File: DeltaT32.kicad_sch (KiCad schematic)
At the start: 35 parts, among them J1 PH2.0, J2 USB_C_Receptacle_USB2.0_16P, J3 SH1.0, Q1 AO3401A, SW1 Boot, SW2 Reset, SW3 SW_SPDT_312, U1 TP4057, U2 MPU-6050, U3 ESP32-C3-MINI-1, U4 AP2112K-3.3

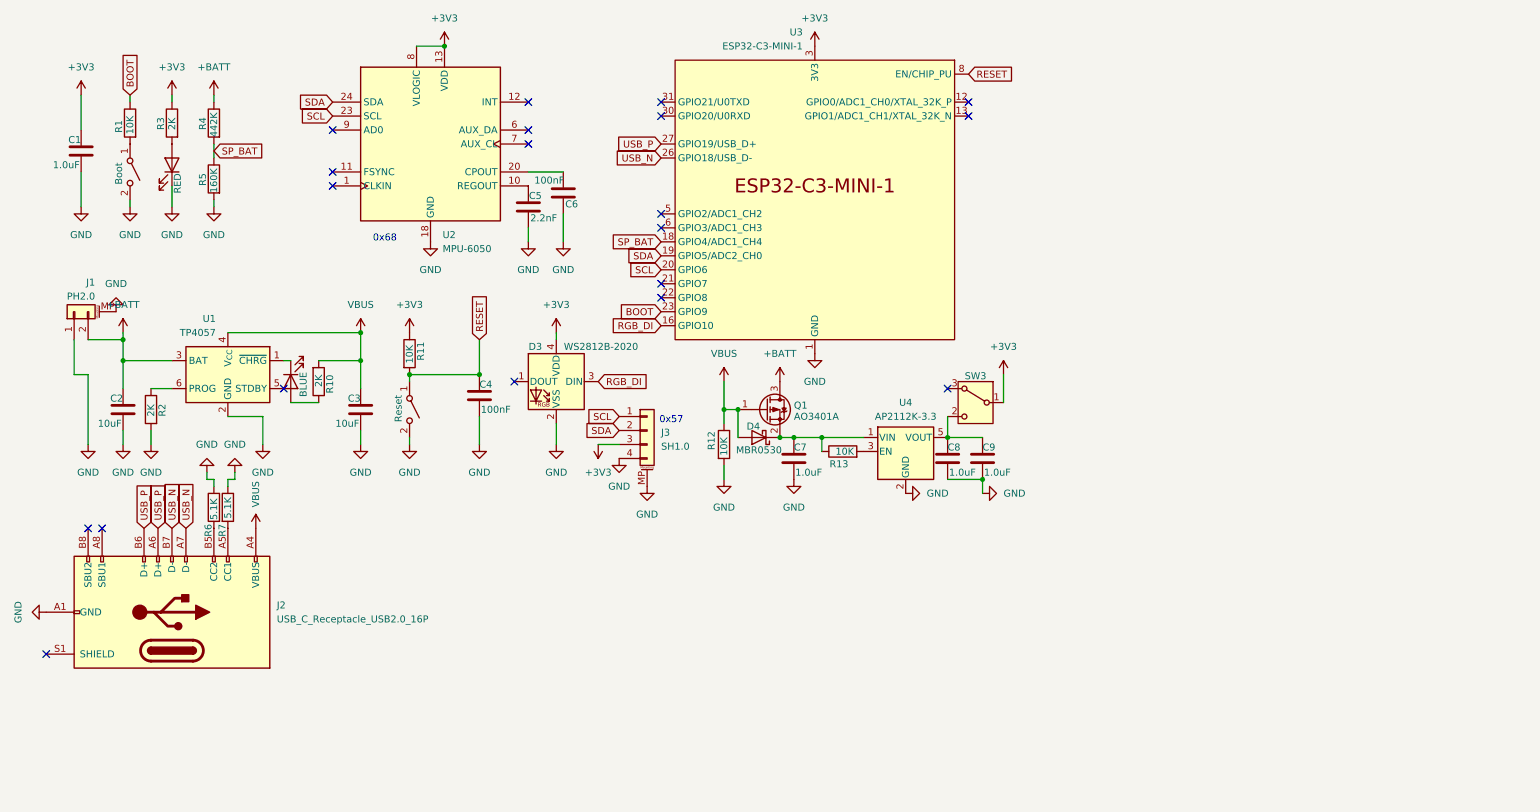
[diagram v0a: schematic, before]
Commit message: Update Board
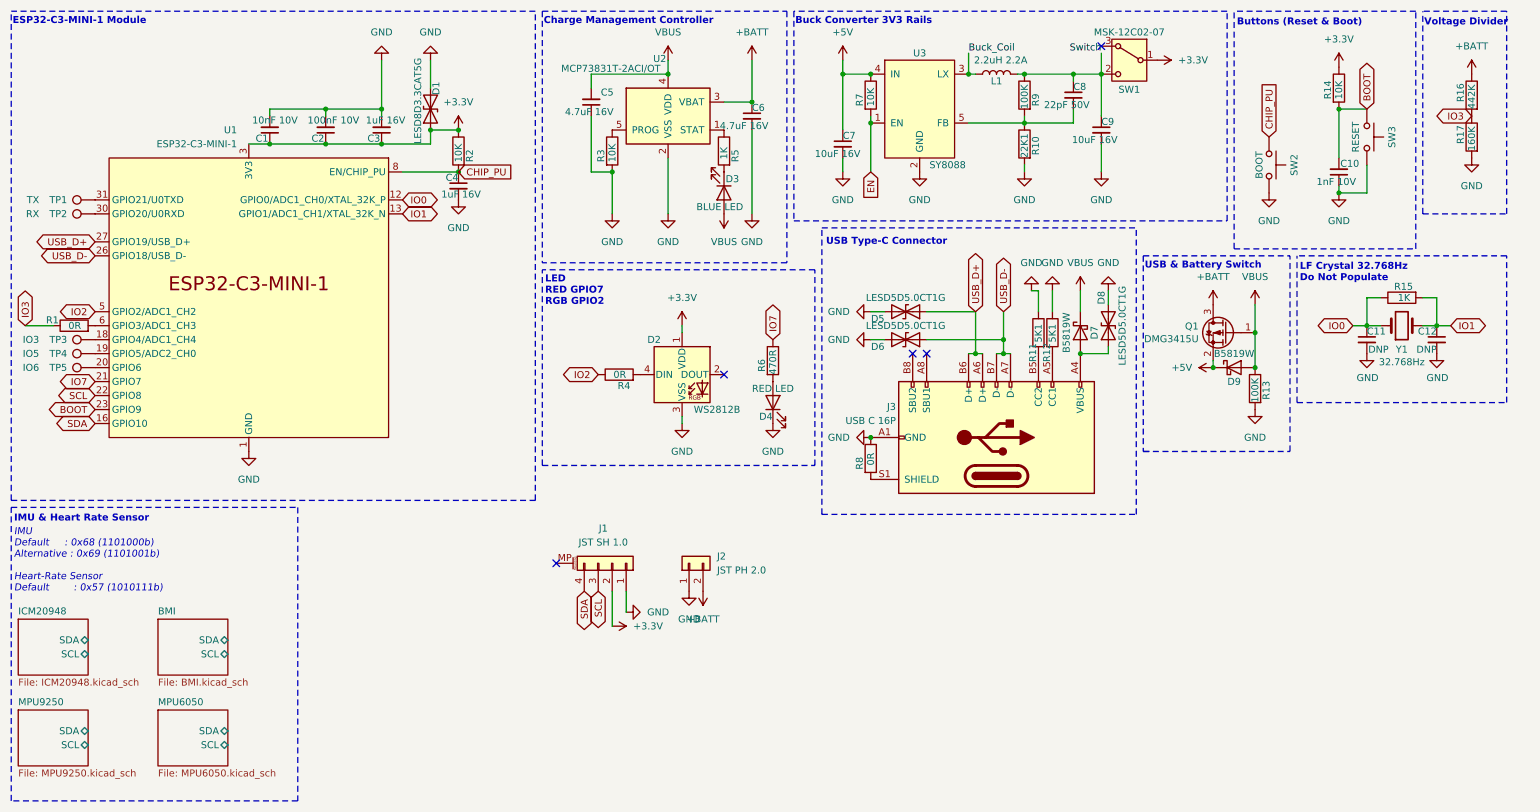
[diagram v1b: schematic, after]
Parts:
- removed C1, C7, C8, C9: 1.0uF, Capacitor_SMD:C_0402_1005Metric, symbol Device:C
- removed C2, C3: 10uF, Capacitor_SMD:C_0402_1005Metric, symbol Device:C
- removed C4, C6: 100nF, Capacitor_SMD:C_0402_1005Metric, symbol Device:C
- removed C5: 2.2nF, Capacitor_SMD:C_0603_1608Metric, symbol Device:C
- removed D1: RED, LED_SMD:LED_0402_1005Metric, symbol Device:LED
- removed D2: BLUE, LED_SMD:LED_0402_1005Metric, symbol Device:LED
- removed D3: WS2812B-2020, LED_SMD:LED_WS2812B-2020_PLCC4_2.0x2.0mm, symbol LED:WS2812B-2020
- removed D4: MBR0530, Diode_SMD:D_SOD-123, symbol Diode:MBR0530
- removed J1: PH2.0, Connector_JST:JST_PH_B2B-PH-SM4-TB_1x02-1MP_P2.00mm_Vertical, symbol Connector_Generic_MountingPin:Conn_01x02_MountingPin
- removed J3: SH1.0, Connector_JST:JST_SH_BM04B-SRSS-TB_1x04-1MP_P1.00mm_Vertical, symbol Connector_Generic_MountingPin:Conn_01x04_MountingPin
- removed Q1: AO3401A, Package_TO_SOT_SMD:SOT-23, symbol Transistor_FET:AO3401A
- removed R11, R12: 10K, Resistor_SMD:R_0402_1005Metric, symbol Device:R
- removed SW1: Boot, Button_Switch_SMD:SW_Push_SPST_NO_Alps_SKRK, symbol Switch:SW_SPST
- removed SW2: Reset, Button_Switch_SMD:SW_Push_SPST_NO_Alps_SKRK, symbol Switch:SW_SPST
- removed SW3: SW_SPDT_312, Button_Switch_SMD:SW_SPDT_PCM12, symbol Switch:SW_SPDT_312
- removed U1: TP4057, Package_TO_SOT_SMD:TSOT-23-6, symbol Battery_Management:TP4057
- removed U2: MPU-6050, Sensor_Motion:InvenSense_QFN-24_4x4mm_P0.5mm, symbol Sensor_Motion:MPU-6050
- removed U3: ESP32-C3-MINI-1, PCM_Espressif:ESP32-C3-MINI-1, symbol PCM_Espressif:ESP32-C3-MINI-1
- removed U4: AP2112K-3.3, Package_TO_SOT_SMD:SOT-23-5, symbol Regulator_Linear:AP2112K-3.3
- added C1: 10nF 10V, Capacitor_SMD:C_0402_1005Metric, symbol Device:C_Small
- added C10: 1nF 10V, Capacitor_SMD:C_0402_1005Metric, symbol Device:C_Small
- added C11, C12: DNP, Capacitor_SMD:C_0402_1005Metric, symbol Device:C_Small
- added C2: 100nF 10V, Capacitor_SMD:C_0402_1005Metric, symbol Device:C_Small
- added C3, C4: 1uF 16V, Capacitor_SMD:C_0402_1005Metric, symbol Device:C_Small
- added C5, C6: 4.7uF 16V, Capacitor_SMD:C_0603_1608Metric, symbol Device:C_Small
- added C7, C9: 10uF 16V, Capacitor_SMD:C_0805_2012Metric, symbol Device:C_Small
- added C8: 22pF 50V, Capacitor_SMD:C_0603_1608Metric, symbol Device:C_Small
- added D1: LESD8D3.3CAT5G, Diode_SMD:D_SOD-882, symbol Device:D_TVS
- added D2: WS2812B, LED_SMD:LED_WS2812B-2020_PLCC4_2.0x2.0mm, symbol LED:WS2812B
- added D3: BLUE LED, LED_SMD:LED_0603_1608Metric, symbol Device:LED
- added D4: RED LED, LED_SMD:LED_0603_1608Metric, symbol Device:LED
- added D5, D6, D8: LESD5D5.0CT1G, Diode_SMD:D_SOD-523, symbol Device:D_TVS
- added D7, D9: B5819W, Diode_SMD:D_SOD-123, symbol Device:D_Schottky
- added J1: JST SH 1.0, Connector_JST:JST_SH_SM04B-SRSS-TB_1x04-1MP_P1.00mm_Horizontal, symbol Connector_Generic_MountingPin:Conn_01x04_MountingPin
- added J2: JST PH 2.0, Connector_JST:JST_PH_B2B-PH-K_1x02_P2.00mm_Vertical, symbol Connector_Generic:Conn_01x02
- added L1: 2.2uH 2.2A, Inductor_SMD:L_Bourns-SRN4018, symbol Device:L
- added Q1: DMG3415U, Package_TO_SOT_SMD:SOT-23, symbol Transistor_FET:DMG2301L
- added R14, R7: 10K, Resistor_SMD:R_0402_1005Metric, symbol Device:R
- added R15, R5: 1K, Resistor_SMD:R_0402_1005Metric, symbol Device:R
- added R4, R8: 0R, Resistor_SMD:R_0402_1005Metric, symbol Device:R
- added R6: 470R, Resistor_SMD:R_0402_1005Metric, symbol Device:R
- added R9: 100K, Resistor_SMD:R_0402_1005Metric, symbol Device:R
- added SW1: MSK-12C02-07, Button_Switch_SMD:SW_SPDT_PCM12, symbol Switch:SW_SPDT_312
- added SW2: BOOT, Button_Switch_SMD:SW_Push_SPST_NO_Alps_SKRK, symbol Switch:SW_Push
- added SW3: RESET, Button_Switch_SMD:SW_Push_SPST_NO_Alps_SKRK, symbol Switch:SW_Push
- added TP1: TX, TestPoint:TestPoint_Pad_D1.0mm, symbol Connector:TestPoint
- added TP2: RX, TestPoint:TestPoint_Pad_D1.0mm, symbol Connector:TestPoint
- added TP3: IO3, TestPoint:TestPoint_Pad_D1.0mm, symbol Connector:TestPoint
- added TP4: IO5, TestPoint:TestPoint_Pad_D1.0mm, symbol Connector:TestPoint
- added TP5: IO6, TestPoint:TestPoint_Pad_D1.0mm, symbol Connector:TestPoint
- added U1: ESP32-C3-MINI-1, PCM_Espressif:ESP32-C3-MINI-1, symbol PCM_Espressif:ESP32-C3-MINI-1
- added U2: MCP73831T-2ACI/OT, Package_TO_SOT_SMD:SOT-23-5, symbol Battery_Management:MCP73831-2-OT
- added U3: SY8088, Package_TO_SOT_SMD:SOT-23-5, symbol Rust_Board:SY8088
- added Y1: 32.768Hz, Crystal:Crystal_SMD_3215-2Pin_3.2x1.5mm, symbol Device:Crystal
- J3: renamed from J2; value USB_C_Receptacle_USB2.0_16P -> USB C 16P; footprint Connector_USB:USB_C_Receptacle_GCT_USB4110 -> Connector_USB:USB_C_Receptacle_GCT_USB4105-xx-A_16P_TopMnt_Horizontal
- R1: value 10K -> 0R
- R10: value 2K -> 22K1
- R11: renamed from R6; value 5.1K -> 5K1
- R12: renamed from R7; value 5.1K -> 5K1
- R13: value 10K -> 100K
- R2, R3: value 2K -> 10K
- renumbered R4 to R16, R5 to R17
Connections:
- net +BATT: now also C6.1, J2.2 (Pin_2), Q1.3 (D), U2.3 (VBAT)
- net BOOT: now also C10.2, R14.2, SW3.1, U1.23 (GPIO9); no longer R1.1
- net GND: now also R10.2, R13.2, R3.2, C1.2, C10.1, C11.2, C12.2, C2.2, C3.2, C4.2, C5.1, C6.2, C7.2, C9.2, D1.2 (A2), D2.3 (VSS), D4.1 (K), D5.2 (A2), D6.2 (A2), D8.2 (A2), J1.1 (Pin_1), J2.1 (Pin_1), R8.1, SW2.2, SW3.2, U1.1 (GND), U1.11 (GND), U1.14 (GND), U1.2 (GND), U1.36 (GND), U1.37 (GND), U1.38 (GND), U1.39 (GND), U1.40 (GND), U1.41 (GND), U1.42 (GND), U1.43 (GND), U1.44 (GND), U1.45 (GND), U1.46 (GND), U1.47 (GND), U1.48 (GND), U1.49 (GND), U1.50 (GND), U1.51 (GND), U1.52 (GND), U1.53 (GND), U2.2 (VSS), U3.2 (GND); no longer R2.2
- net SCL: now also J1.3 (Pin_3), U1.22 (GPIO8)
- net SDA: now also J1.4 (Pin_4), U1.16 (GPIO10)
- net VBUS: now also R13.1, C5.2, D3.2 (A), D7.1 (K), D9.2 (A), Q1.1 (G), U2.4 (VDD); no longer J3.A4 (VBUS), J3.A9 (VBUS), J3.B4 (VBUS), J3.B9 (VBUS), R10.2
- net +3.3V: now reaches R2.1
- net +3.3V: now also C1.1, C2.1, C3.1, D1.1 (A1), D2.1 (VDD), J1.2 (Pin_2), R14.1, SW1.1 (B), U1.3 (3V3)
- net at R1.2: now also U1.6 (GPIO3/ADC1_CH3)
- net at R10.1: now also C8.2, R9.2, U3.5 (FB)
- net at J3.S1 (SHIELD): now also R8.2
- net +3V3: no longer names the net of R3.1
- net +3V3: now also U2.5 (PROG)
- net SP_BAT renamed IO3
- net IO3: now also R1.1
- net USB_N renamed USB_D-
- net USB_D-: now also D6.1 (A1), U1.26 (GPIO18/USB_D-)
- net USB_P renamed USB_D+
- net USB_D+: now also D5.1 (A1), U1.27 (GPIO19/USB_D+)
- new net: TP3.1, U1.18 (GPIO4/ADC1_CH4)
- new net: R5.1, U2.1 (STAT)
- new net: D3.1 (K), R5.2
- new net: D7.2 (A), D8.1 (A1), J3.A4 (VBUS), J3.A9 (VBUS), J3.B4 (VBUS), J3.B9 (VBUS)
- new net: D2.4 (DIN), R4.2
- new net: TP4.1, U1.19 (GPIO5/ADC2_CH0)
- new net: TP5.1, U1.20 (GPIO6)
- new net: TP2.1, U1.30 (GPIO20/U0RXD)
- new net: TP1.1, U1.31 (GPIO21/U0TXD)
- new net: D4.2 (A), R6.2
- new net +5V: C7.1, D9.1 (K), Q1.2 (S), R7.1, U3.4 (IN)
- new net Buck_Coil: L1.1, U3.3 (LX)
- new net CHIP_PU: C4.1, R2.2, SW2.1, U1.8 (EN/CHIP_PU)
- new net EN: R7.2, U3.1 (EN)
- new net IO0: C11.1, R15.1, U1.12 (GPIO0/ADC1_CH0/XTAL_32K_P), Y1.1
- new net IO1: C12.1, R15.2, U1.13 (GPIO1/ADC1_CH1/XTAL_32K_N), Y1.2
- new net IO2: R4.1, U1.5 (GPIO2/ADC1_CH2)
- new net IO7: R6.1, U1.21 (GPIO7)
- new net Switch: C8.1, C9.1, L1.2, R9.1, SW1.2 (C)
- no-connect marks 20 -> 5
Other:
- added sheet BMI (BMI.kicad_sch)
- added sheet ICM20948 (ICM20948.kicad_sch)
- added sheet MPU6050 (MPU6050.kicad_sch)
- added sheet MPU9250 (MPU9250.kicad_sch)
- note added: "Buck Converter 3V3 Rails"
- note added: "Buttons (Reset & Boot)"
- note added: "Charge Management Controller"
- note added: "ESP32-C3-MINI-1 Module"
- note added: "IMU & Heart Rate Sensor"
- note added: "IMU Default : 0x68 (1101000b) Alternative : 0x69 (1101001b) Heart-Rate Sensor Default : 0x57 (1010111b)"
- note added: "LED RED GPIO7 RGB GPIO2"
- note added: "LF Crystal 32.768Hz Do Not Populate"
- note added: "USB & Battery Switch"
- note added: "USB Type-C Connector"
- note added: "Voltage Divider"
- title: (none) -> DeltaT32
- moved on the sheet: J3, R11, R12, R16, R17

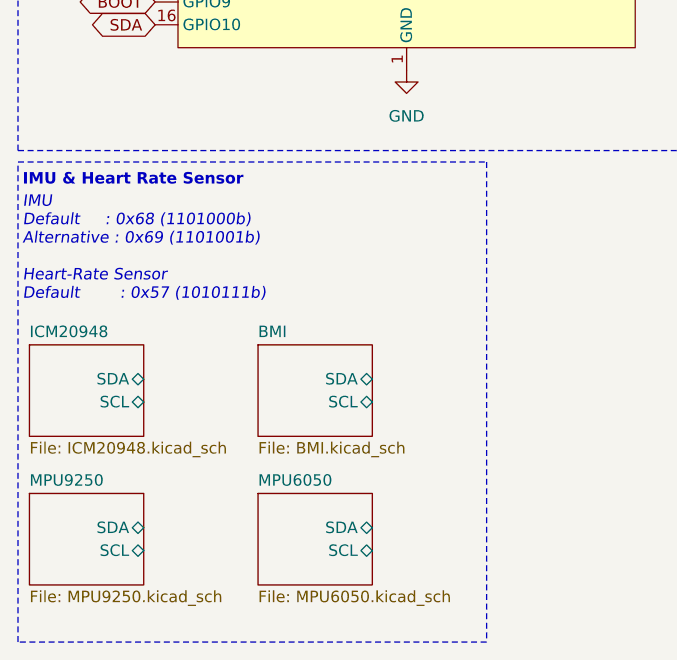
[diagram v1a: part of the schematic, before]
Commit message: Update Board
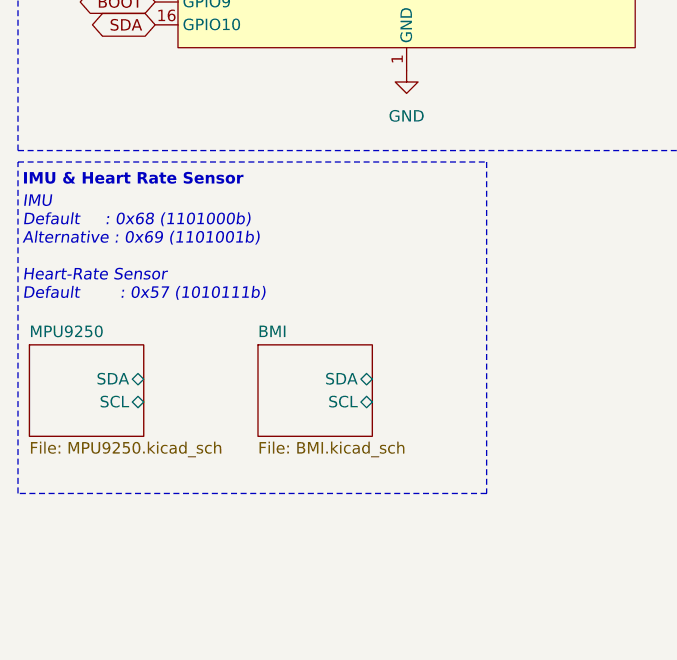
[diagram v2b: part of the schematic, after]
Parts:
- J2: footprint Connector_JST:JST_PH_B2B-PH-K_1x02_P2.00mm_Vertical -> Connector_JST:JST_PH_S2B-PH-K_1x02_P2.00mm_Horizontal
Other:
- removed sheet ICM20948
- removed sheet MPU6050
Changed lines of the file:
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@@
 	(polyline
 		(pts
-			(xy 64.77 102.87) (xy 64.77 156.21)
+			(xy 64.77 102.87) (xy 64.77 139.7)
 		)
 		(stroke
@@
 	(polyline
 		(pts
-			(xy 12.7 156.21) (xy 12.7 102.87)
+			(xy 12.7 139.7) (xy 12.7 102.87)
 		)
 		(stroke
@@
 	(polyline
 		(pts
-			(xy 64.77 156.21) (xy 12.7 156.21)
+			(xy 64.77 139.7) (xy 12.7 139.7)
 		)
 		(stroke
@@
 			"AAAAAAAAAAAAAAAAAAAAAAAAAAAAAAAAAAAAAAAAAAAAAAAAAAAAAADwAAAAAAAAAASzwJEABACA"
 			"0JgX/psBAACAvxj+mwEAAIC/GP6bAQAAABAAAAAAAAAAAAAAAAAAAICvGP6bAQAAAAAAAAAAAAAA"
-			"AAAAAAAAAAAAAAAAAAAAoK8Y/psBAAAAAAAAAAAAAAAAAAAAAAAAAAAAAAAAAADArxj+mw=="
+			"AAAAAAAAAAAAAAAAAAAAoK8Y/psBAAAAAAAAAAAAAAAAAAAAAAAAAAAAAAAAAADArxj+mwAAAAAA"
+			"AAAAAAAAAAAAAAAAAAAAAAAAAAAAAAAAAAAAAAAAAAAAAAAAAAAAAAAAAAAAAAAAAAAAAAAAAAAA"
+			"AAAAAAAAAAAAAAAAAAAAAAAAAAAAAAAAAAAAAAAAAAAAAAAAAAAAAAAAAAAAAAAAAAAAAAAAAAAA"
+			"AAAAAAAAAAAAAAAAAAAAAAAAAAAAAAAAAAAAAAAAAAAAAAAAAAAAAAAAAAAAAAAAAAAAAAAAAAAA"
+			"AAAAAAAAAAAAAAAAAAAAAAAAAAAAAAAAAAAAAAAAAAAAAAAAAAAAAAAAAAAAAAAAAAAAAAAAAAAA"
+			"AAAAAAAAAAAAAAAAAAAAAAAAAAAAAAAAAAAAAAAAAAAAAAAAAAAAAAAAAAAAAAAAAAAAAAAAAAAA"
+			"AAAAAAAAAAAAAAAAAAAAAAAAAAAAAAAAAAAAAAAAAAAAAAAAAAAAAAAAAAAAAAAAAAAAAAAAAAAA"
+			"AAAAAAAAAAAAAAAAAAAAAAAAAAAAAAAAAAAAAAAAAAAAAAAAAAAAAAAAAAAAAAAAAAAAAAAAAAAA"
+			"AAAAAAAAAAAAAAAAAAAAAAAAAAAAAAAAAAAAAAAAAAAAAAAAAAAAAAAAAAAAAAAAAAAAAAAAAAAA"
+			"AAAAAAAAAAAAAAAAAAAAAAAAAAAAAAAAAAAAAAAAAAAAAAAAAAAAAAAAAAAAAAAAAAAAAAAAAAAA"
+			"AAAAAAAAAAAAAAAAAAAAAAAAAAAAAAAAAAAAAAAAAAAAAAAAAAAAAAAAAAAAAAAAAAAAAAAAAAAA"
+			"AAAAAAAAAAAAAAAAAAAAAAAAAAAAAAAAAAAAAAAAAAAAAAAAAAAAAAAAAAAAAAAAAAAAAAAAAAAA"
+			"AAAAAAAAAAAAAAAAAAAAAAAAAAAAAAAAAAAAAAAAAAAAAAAAAAAAAAAAAAAAAAAAAAAAAAAAAAAA"
+			"AAAAAAAAAAAAAAAAAAAAAAAAAAAAAAAAAAAAAAAAAAAAAAAAAAAAAAAAAAAAAAAAAAAAAAAAAAAA"
+			"AAAAAAAAAAAAAAAAAAAAAAAAAAAAAAAAAAAAAAAAAAAAAAAAAAAAAAAAAAAAAAAAAAAAAAAAAAAA"
+			"AAAAAAAAAAAAAAAAAAAAAAAAAAAAAAAAAAAAAAAAAAAAAAAAAAAAAAAAAAAAAAAAAAAAAAAAAAAA"
+			"AAAAAAAAAAAAAAAAAAAAAAAAAAAAAAAAAAAAAAAAAAAAAAAAAAAAAAAAAAAAAAAAAAAAAAAAAAAA"
+			"AAAAAAAAAAAAAAAAAAAAAAAAAAAAAAAAAAAAAAAAAAAAAAAAAAAAAAAAAAAAAAAAAAAAAAAAAAAA"
+			"AAAAAAAAAAAAAAAAAAAAAAAAAAAAAAAAAAAAAAAAAAAAAAAAAAAAAAAAAAAAAAAAAAAAAAAAAAAA"
+			"AAAAAAAAAAAAAAAAAAAAAAAAAAAAAAAAAAAAAAAAAAAAAAAAAAAAAAAAAAAAAAAAAAAAAAAAAAAA"
+			"AAAAAAAAAAAAAAAAAAAAAAAAAAAAAAAAAAAAAAAAAAAAAAAAAAAAAAAAAAAAAAAAAAAAAAAAAAAA"
+			"AAAAAAAAAAAAAAAAAAAAAAAAAAAAAAAAAAAAAAAAAAAAAAAAAAAAAAAAAAAAAAAAAAAAAAAAAAAA"
+			"AAAAAAAAAAAAAAAAAAAAAAAAAAAAAAAAAAAAAAAAAAAAAAAAAAAAAAAAAAAAAAAAAAAAAAAAAAAA"
+			"AAAAAAAAAAAAAAAAAAAAAAAAAAAAAAAAAAAAAAAAAAAAAAAAAAAAAAAAAAAAAAAAAAAAAAAAAAAA"
+			"AAAAAAAAAAAAAAAAAAAAAAAAAAAAAAAAAAAAAAAAAAAAAAAAAAAAAAAAAAAAAAAAAAAAAAAAAAAA"
+			"AAAAAAAAAAAAAAAAAAAAAAAAAAAAAAAAAAAAAAAAAAAAAAAAAAAAAAAAAAAAAAAAAAAAAAAAAAAA"
+			"AAAAAAAAAAAAAAAAAAAAAAAAAAAAAAAAAAAAAAAAAAAAAAAAAAAAAAAAAAAAAAAAAAAAAAAAAAAA"
+			"AAAAAAAAAAAAAAAAAAAAAAAAAAAAAAAAAAAAAAAAAAAAAAAAAAAAAAAAAAAAAAAAAAAAAAAAAAAA"
+			"AAAAAAAAAAAAAAAAAAAAAAAAAAAAAAAAAAAAAAAAAAAAAAAAAAAAAAAAAAAAAAAAAAAAAAAAAAAA"
+			"AAAAAAAAAAAAAAAAAAAAAAAAAAAAAAAAAAAAAAAAAAAAAAAAAAAAAAAAAAAAAAAAAAAAAAAAAAAA"
+			"AAAAAAAAAAAAAAAAAAAAAAAAAAAAAAAAAAAAAAAAAAAAAAAAAAAAAAAAAAAAAAAAAAAAAAAAAAAA"
+			"AAAAAAAAAAAAAAAAAAAAAAAAAAAAAAAAAAAAAAAAAAAAAAAAAAAAAAAAAAAAAAAAAAAAAAAAAAAA"
+			"AAAAAAAAAAAAAAAAAAAAAAAAAAAAAAAAAAAAAAAAAAAAAAAAAAAAAAAAAAAAAAAAAAAAAAAAAAAA"
+			"AAAAAAAAAAAAAAAAAAAAAAAAAAAAAAAAAAAAAAAAAAAAAAAAAAAAAAAAAAAAAAAAAAAAAAAAAAAA"
+			"AAAAAAAAAAAAAAAAAAAAAAAAAAAAAAAAAAAAAAAAAAAAAAAAAAAAAAAAAAAAAAAAAAAAAAAAAAAA"
+			"AAAAAAAAAAAAAAAAAAAAAAAAAAAAAAAAAAAAAAAAAAAAAAAAAAAAAAAAAAAAAAAAAAAAAAAAAAAA"
+			"AAAAAAAAAAAAAAAAAAAAAAAAAAAAAAAAAAAAAAAAAAAAAAAAAAAAAAAAAAAAAAAAAAAAAP///wQA"
+			"AAD4/////////3gDAAAAAAAA/////wQAAAD4/////////wAAAAAAAAAA/////wQAAAD4////////"
+			"/94AAAAAAAAA/////wQAAAD4/////////98CAAAAAAAA/////wQAAAD4/////////2gBAAAAAAAA"
+			"/////wQAAAD4/////////wAAAAAAAAAA/////wQAAAD4/////////xsDAAAAAAAA/////wQAAAD4"
+			"/////////70AAAAAAAAA/////wQAAAD4/////////6IBAAAAAAAA/////wQAAAD4/////////9gA"
+			"AAAAAAAA/////wQAAAD4/////////w8BAAAAAAAA/////wQAAAD4/////////0EAAAAAAAAA////"
+			"/wQAAAD4/////////5oAAAAAAAAA/////wQAAAD4/////////wAAAAAAAAAA/////wQAAAD4////"
+			"/////wAAAAAAAAAA/////wQAAAD4/////////wAAAAAAAAAA/////wQAAAD4/////////5gAAAAA"
+			"AAAA/////wQAAAD4/////////wAAAAAAAAAA/////wQAAAD4/////////9ICAAAAAAAA/////wQA"
+			"AAD4/////////18AAAAAAAAA/////wQAAAD4/////////9kBAAAAAAAA/////wQAAAD4////////"
+			"/xwBAAAAAAAA/////wQAAAD4/////////0sAAAAAAAAA/////wQAAAD4/////////wAAAAAAAAAA"
+			"/////wQAAAD4/////////48AAAAAAAAA/////wQAAAD4/////////wAAAAAAAAAA/////wQAAAD4"
+			"/////////wAAAAAAAAAA/////wQAAAD4/////////wAAAAAAAAAA/////wQAAAD4/////////10A"
+			"AAAAAAAA/////wQAAAD4/////////5wAAAAAAAAA/////wQAAAD4/////////9gCAAAAAAAA////"
+			"/wQAAAD4/////////wAAAAAAAAAA/////wQAAAD4/////////wAAAAAAAAAA/////wQAAAD4////"
+			"/////wAAAAAAAAAA/////wQAAAD4/////////wAAAAAAAAAA/////wQAAAD4/////////wAAAAAA"
+			"AAAA/////wQAAAD4/////////zoBAAAAAAAA/////wQAAAD4/////////0sCAAAAAAAA/////wQA"
+			"AAD4/////////8wAAAAAAAAA/////wQAAAD4//////////kCAAAAAAAA/////wQAAAD4////////"
+			"/9QBAAAAAAAA/////wQAAAD4/////////wAAAAAAAAAA/////wQAAAD4/////////wAAAP9aWlr/"
+			"Wlpa/1paWv9aWlr/Wlpa/1paWv9aWlr/Wlpa/1paWv9aWlr/Wlpa/1paWv9aWlr/Wlpa/1paWv9a"
+			"Wlr/Wlpa/1paWv9aWlr/Wlpa/1paWv9aWlr/Wlpa/1paWv9aWlr/Wlpa/1paWv9aWlr/Wlpa/1pa"
+			"Wv9aWlr/Wlpa/1paWv9aWlr/Wlpa/1paWv9aWlr/Wlpa/1paWv9aWlr/Wlpa/1paWv9aWlr/Wlpa"
+			"/1paWv9aWlr/Wlpa/1paWv9aWlr/Wlpa/1paWv9aWlr/Wlpa/1paWv+inIz/0MWs/9DFrP/Qxaz/"
+			"0MWs/9DFrP/Qxaz/0MWs/9DFrP/Qxaz/0MWs/9DFrP/Qxaz/0MWs/9DFrP/Qxaz/0MWs/9DFrP/Q"
+			"xaz/0MWs/9DFrP/Qxaz/0MWs/9DFrP/Qxaz/0MWs/9DFrP/Qxaz/0MWs/9DFrP/Qxaz/0MWs/9DF"
+			"rP/Qxaz/0MWs/9DFrP/Qxaz/0MWs/9DFrP/Qxaz/0MWs/9DFrP/Qxaz/0MWs/9DFrP/Qxaz/0MWs"
+			"/9DFrP/Qxaz/0MWs/9DFrP/Qxaz/0MWs/9DFrP/Qxaz/0MWs/9DFrP/Qxaz/0MWs/9DFrP/Qxaz/"
+			"0MWs/9DFrP/Qxaz/0MWs/9DFrP/Qxaz/0MWs/9DFrP/Qxaz/0MWs/9DFrP/Qxaz/0MWs/9DFrP/Q"
+			"xaz/0MWs/9DFrP/Qxaz/0MWs/9DFrP/Qxaz/0MWs/9DFrP/Qxaz/0MWs/9DFrP/Qxaz/0MWs/9DF"
+			"rP/Qxaz/0MWs/9DFrP/Qxaz/0MWs/9DFrP/Qxaz/0MWs/9DFrP/Qxaz/0MWs/9DFrP/Qxaz/0MWs"
+			"/9DFrP/Qxaz/0MWs/9DFrP/Qxaz/0MWs/9DFrP/Qxaz/0MWs/9DFrP/Qxaz/0MWs/9DFrP/Qxaz/"
+			"0MWs/9DFrP/Qxaz/0MWs/9DFrP/Qxaz/0MWs/9DFrP/Qxaz/vbOd/zMzM/8zMzP/MzMz/zMzM/8z"
+			"MzP/MzMz/zMzM/8zMzP/MzMz/zMzM/8zMzP/MzMz/zMzM/8zMzP/MzMz/zMzM/8zMzP/MzMz/zMz"
+			"M/8zMzP/MzMz/zMzM/8zMzP/SUdE/6CZh//Qxaz/0MWs/9DFrP/Qxaz/0MWs/9DFrP/Qxaz/0MWs"
+			"/9DFrP/Qxaz/0MWs/9DFrP/Qxaz/0MWs/9DFrP/Topv/4RBS/9wfV//gFlT/0L+p/9DFrP/Qxaz/"
+			"0MWs/9DFrP/Qxaz/0MWs/9DFrP/Qxaz/0MWs/9DFrP/Qxaz/0MWs/9DFrP/Qxaz/0MWs/9DFrP/Q"
+			"xaz/0MWs/9DFrP/Kv6j/bWtn/1paWv9aWlr/Wlpa/1paWv9aWlr/Wlpa/1paWv9aWlr/Wg=="
 		)
 	)
@@
 			)
 		)
-		(property "Footprint" "Connector_JST:JST_PH_B2B-PH-K_1x02_P2.00mm_Vertical"
+		(property "Footprint" "Connector_JST:JST_PH_S2B-PH-K_1x02_P2.00mm_Horizontal"
 			(at 135.89 113.03 0)
 			(effects
@@
 	)
 	(sheet
-		(at 13.97 123.19)
-		(size 12.7 10.16)
-		(exclude_from_sim no)
-		(in_bom yes)
-		(on_board yes)
-		(dnp no)
-		(fields_autoplaced yes)
-		(stroke
-			(width 0.1524)
-			(type solid)
-		)
-		(fill
-			(color 0 0 0 0.0000)
-		)
-		(property "Sheetname" "ICM20948"
-			(at 13.97 122.4784 0)
-			(effects
-				(font
-					(size 1.27 1.27)
-				)
-				(justify left bottom)
-			)
-		)
-		(property "Sheetfile" "ICM20948.kicad_sch"
-			(at 13.97 133.9346 0)
-			(effects
-				(font
-					(size 1.27 1.27)
-				)
-				(justify left top)
-			)
-		)
-		(pin "SDA" bidirectional
-			(at 26.67 127 0)
-			(effects
-				(font
-					(size 1.27 1.27)
-				)
-				(justify right)
-			)
-		)
-		(pin "SCL" bidirectional
-			(at 26.67 129.54 0)
-			(effects
-				(font
-					(size 1.27 1.27)
-				)
-				(justify right)
-			)
-		)
-		(instances
-			(project "DeltaT32"
-				(path "/418142f0-ca8b-4509-a0db-baeccce9fb59"
-					(page "2")
-				)
-			)
-		)
-	)
-	(sheet
-		(at 39.37 139.7)
-		(size 12.7 10.16)
-		(exclude_from_sim no)
-		(in_bom yes)
-		(on_board yes)
-		(dnp no)
-		(fields_autoplaced yes)
-		(stroke
-			(width 0.1524)
-			(type solid)
-		)
-		(fill
-			(color 0 0 0 0.0000)
-		)
-		(property "Sheetname" "MPU6050"
-			(at 39.37 138.9884 0)
-			(effects
-				(font
-					(size 1.27 1.27)
-				)
-				(justify left bottom)
-			)
-		)
-		(property "Sheetfile" "MPU6050.kicad_sch"
-			(at 39.37 150.4446 0)
-			(effects
-				(font
-					(size 1.27 1.27)
-				)
-				(justify left top)
-			)
-		)
-		(pin "SDA" bidirectional
-			(at 52.07 143.51 0)
-			(effects
-				(font
-					(size 1.27 1.27)
-				)
-				(justify right)
-			)
-		)
-		(pin "SCL" bidirectional
-			(at 52.07 146.05 0)
-			(effects
-				(font
-					(size 1.27 1.27)
-				)
-				(justify right)
-			)
-		)
-		(instances
-			(project "DeltaT32"
-				(path "/418142f0-ca8b-4509-a0db-baeccce9fb59"
-					(page "5")
-				)
-			)
-		)
-	)
-	(sheet
 		(at 39.37 123.19)
 		(size 12.7 10.16)
@@
 	)
 	(sheet
-		(at 13.97 139.7)
+		(at 13.97 123.19)
 		(size 12.7 10.16)
 		(exclude_from_sim no)
@@
 		)
 		(property "Sheetname" "MPU9250"
-			(at 13.97 138.9884 0)
+			(at 13.97 122.4784 0)
 			(effects
 				(font
@@
 		)
 		(property "Sheetfile" "MPU9250.kicad_sch"
-			(at 13.97 150.4446 0)
+			(at 13.97 133.9346 0)
 			(effects
 				(font
@@
 		)
 		(pin "SDA" bidirectional
-			(at 26.67 143.51 0)
+			(at 26.67 127 0)
 			(effects
 				(font
@@
 		)
 		(pin "SCL" bidirectional
-			(at 26.67 146.05 0)
+			(at 26.67 129.54 0)
 			(effects
 				(font
